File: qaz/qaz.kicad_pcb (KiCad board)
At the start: 2 copper layers, 223.6 x 57.1 mm, 49 parts, among them J1 OLED-128x32, SW1 SW_Push, SW10 SW_Push, SW11 SW_Push, SW12 SW_Push, SW13 SW_Push, SW14 SW_Push, SW15 SW_Push, SW16 SW_Push, SW17 SW_Push, SW18 SW_Push, SW19 SW_Push, SW2 SW_Push, SW20 SW_Push, SW21 SW_Push, SW22 SW_Push, SW23 SW_Push, SW24 SW_Push, SW25 SW_Push, SW26 SW_Push, SW27 SW_Push, SW28 SW_Push, SW3 SW_Push, SW4 SW_Push, SW5 SW_Push, SW6 SW_Push, SW7 SW_Push, SW8 SW_Push, SW9 SW_Push, U1 rp2040-zero

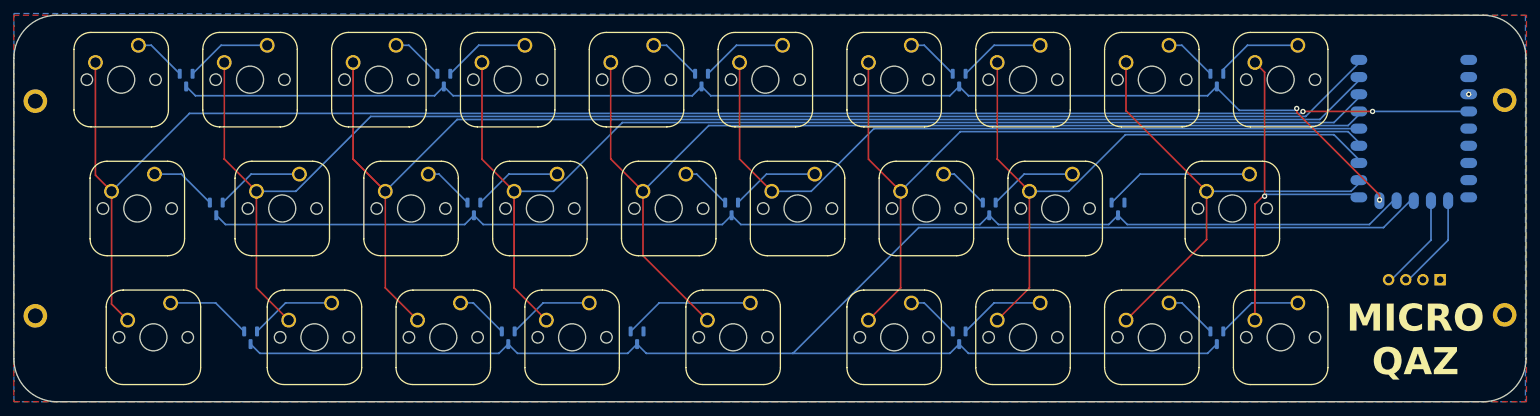
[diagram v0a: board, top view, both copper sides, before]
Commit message: .
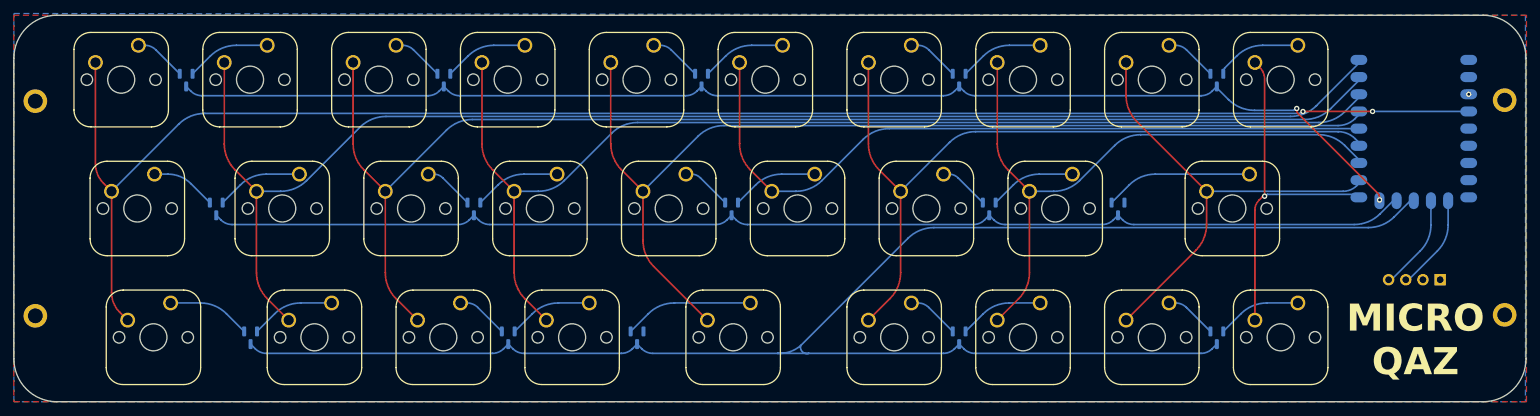
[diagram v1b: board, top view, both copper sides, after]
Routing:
- net r2: track 248.8 -> 251.3 mm
- net r0: track 189.1 -> 187.7 mm
- net c1: track 213.6 -> 212.3 mm
- net c3: track 173.4 -> 172.1 mm
- net c7: track 96.5 -> 95.1 mm
- net r1: track 181.3 -> 180.0 mm
- net c2: track 193.5 -> 192.5 mm
- net c6: track 114.8 -> 113.9 mm
- net c4: track 155.3 -> 154.3 mm
- net c5: track 112.2 -> 111.4 mm
- net c0: track 245.3 -> 244.6 mm
- net c8: track 71.7 -> 71.0 mm
